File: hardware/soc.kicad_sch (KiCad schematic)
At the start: 2 parts, among them U16 MPFS025T-FCVG484E, U4 MPFS025T-FCVG484E

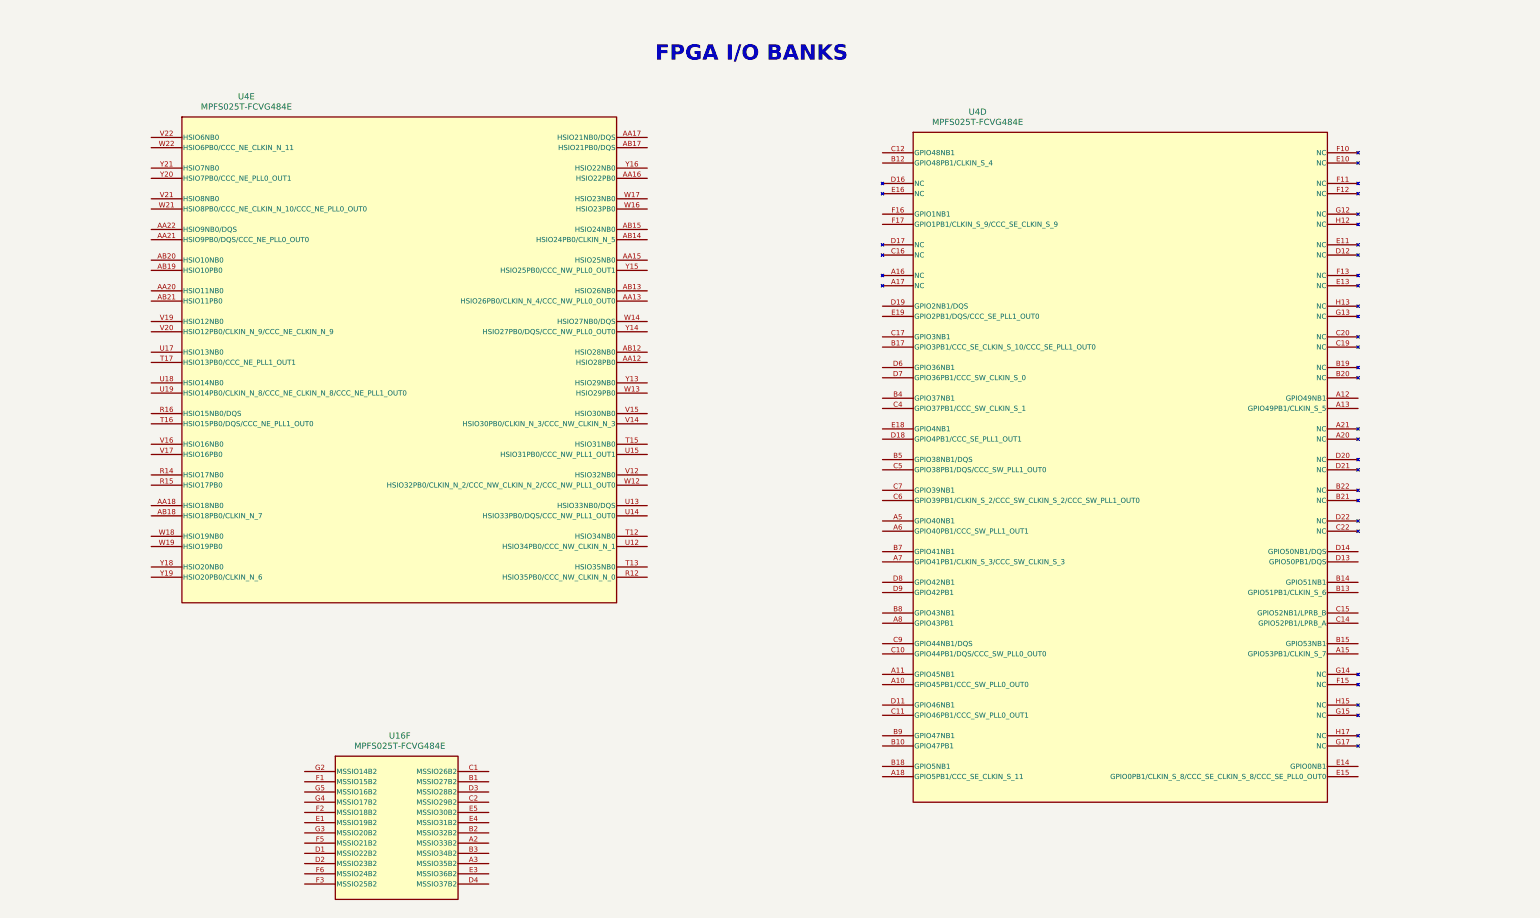
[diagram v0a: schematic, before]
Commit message: need finish io banks pinouts
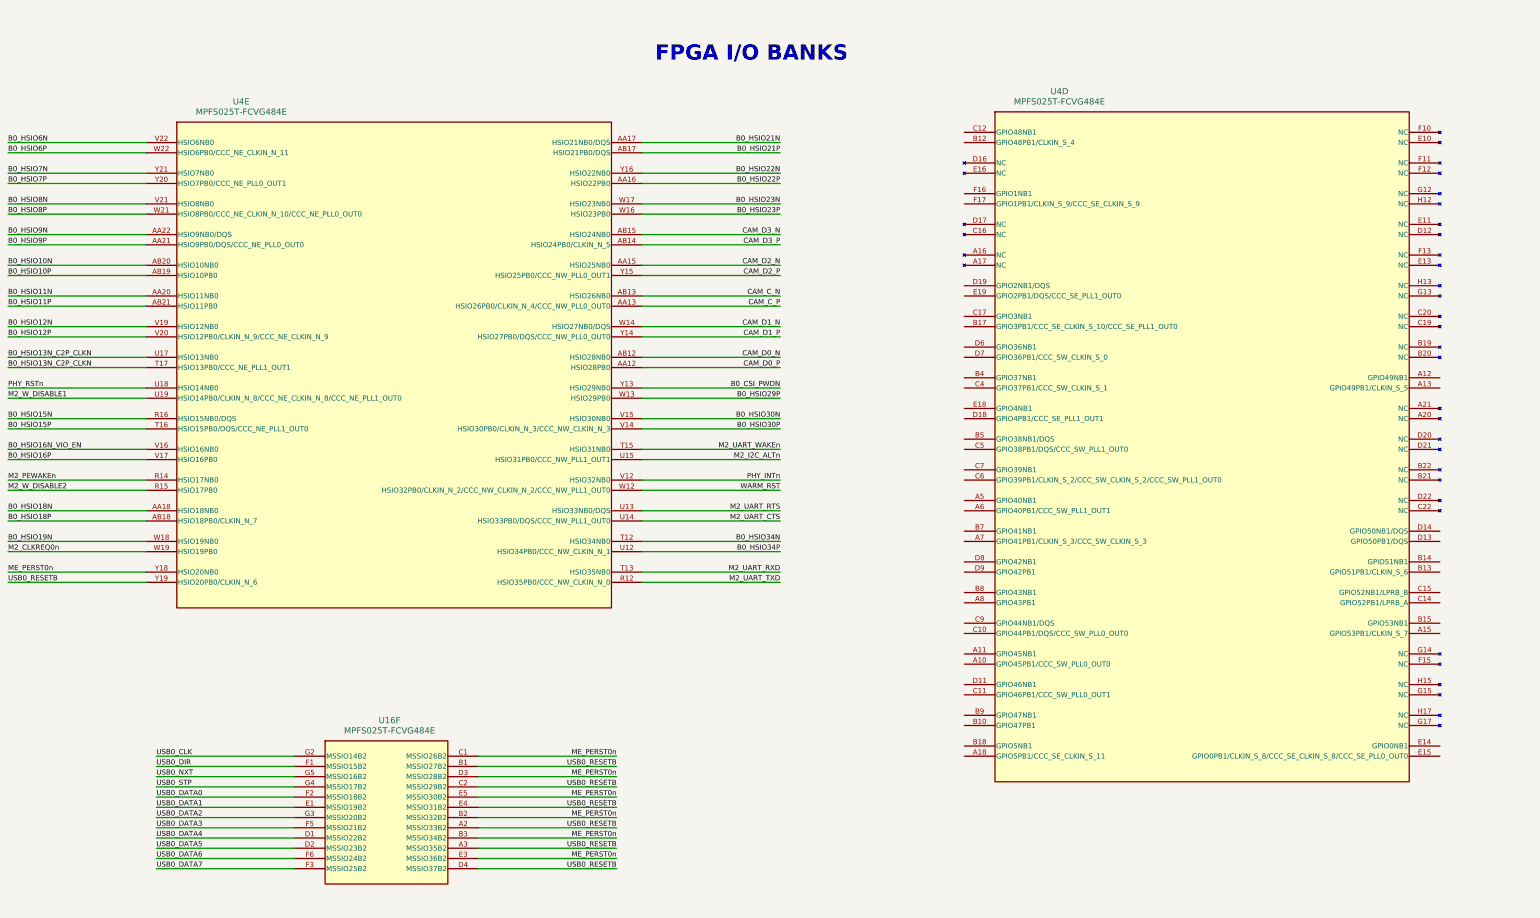
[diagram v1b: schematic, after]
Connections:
- net USB0_RESETB: now reaches U16.A2 (MSSIO33B2)
- net USB0_RESETB: now also U16.A3 (MSSIO35B2), U16.B1 (MSSIO27B2), U16.C2 (MSSIO29B2), U16.D4 (MSSIO37B2), U16.E4 (MSSIO31B2), U4.Y19 (HSIO20PB0/CLKIN_N_6)
- net ME_PERST0n: now reaches U16.B2 (MSSIO32B2)
- net ME_PERST0n: now also U16.B3 (MSSIO34B2), U16.C1 (MSSIO26B2), U16.D3 (MSSIO28B2), U16.E3 (MSSIO36B2), U16.E5 (MSSIO30B2), U4.Y18 (HSIO20NB0)
- net USB0_DATA4: now reaches U16.D1 (MSSIO22B2)
- net USB0_DATA5: now reaches U16.D2 (MSSIO23B2)
- net USB0_DATA1: now reaches U16.E1 (MSSIO19B2)
- net USB0_DIR: now reaches U16.F1 (MSSIO15B2)
- net USB0_DATA0: now reaches U16.F2 (MSSIO18B2)
- net USB0_DATA7: now reaches U16.F3 (MSSIO25B2)
- net USB0_DATA3: now reaches U16.F5 (MSSIO21B2)
- net USB0_DATA6: now reaches U16.F6 (MSSIO24B2)
- net USB0_CLK: now reaches U16.G2 (MSSIO14B2)
- net USB0_DATA2: now reaches U16.G3 (MSSIO20B2)
- net USB0_STP: now reaches U16.G4 (MSSIO17B2)
- net USB0_NXT: now reaches U16.G5 (MSSIO16B2)
- net CAM_D0_P: now reaches U4.AA12 (HSIO28PB0)
- net CAM_C_P: now reaches U4.AA13 (HSIO26PB0/CLKIN_N_4/CCC_NW_PLL0_OUT0)
- net CAM_D2_N: now reaches U4.AA15 (HSIO25NB0)
- net B0_HSIO22P: now reaches U4.AA16 (HSIO22PB0)
- net B0_HSIO21N: now reaches U4.AA17 (HSIO21NB0/DQS)
- net B0_HSIO18N: now reaches U4.AA18 (HSIO18NB0)
- net B0_HSIO11N: now reaches U4.AA20 (HSIO11NB0)
- net B0_HSIO9P: now reaches U4.AA21 (HSIO9PB0/DQS/CCC_NE_PLL0_OUT0)
- net B0_HSIO9N: now reaches U4.AA22 (HSIO9NB0/DQS)
- net CAM_D0_N: now reaches U4.AB12 (HSIO28NB0)
- net CAM_C_N: now reaches U4.AB13 (HSIO26NB0)
- net CAM_D3_P: now reaches U4.AB14 (HSIO24PB0/CLKIN_N_5)
- net CAM_D3_N: now reaches U4.AB15 (HSIO24NB0)
- net B0_HSIO21P: now reaches U4.AB17 (HSIO21PB0/DQS)
- net B0_HSIO18P: now reaches U4.AB18 (HSIO18PB0/CLKIN_N_7)
- net B0_HSIO10P: now reaches U4.AB19 (HSIO10PB0)
- net B0_HSIO10N: now reaches U4.AB20 (HSIO10NB0)
- net B0_HSIO11P: now reaches U4.AB21 (HSIO11PB0)
- net M2_UART_TXD: now reaches U4.R12 (HSIO35PB0/CCC_NW_CLKIN_N_0)
- net M2_PEWAKEn: now reaches U4.R14 (HSIO17NB0)
- net M2_W_DISABLE2: now reaches U4.R15 (HSIO17PB0)
- net B0_HSIO15N: now reaches U4.R16 (HSIO15NB0/DQS)
- net B0_HSIO34N: now reaches U4.T12 (HSIO34NB0)
- net M2_UART_RXD: now reaches U4.T13 (HSIO35NB0)
- net M2_UART_WAKEn: now reaches U4.T15 (HSIO31NB0)
- net B0_HSIO15P: now reaches U4.T16 (HSIO15PB0/DQS/CCC_NE_PLL1_OUT0)
- net B0_HSIO13N_C2P_CLKN: now reaches U4.T17 (HSIO13PB0/CCC_NE_PLL1_OUT1)
- net B0_HSIO13N_C2P_CLKN: now also U4.U17 (HSIO13NB0)
- net B0_HSIO34P: now reaches U4.U12 (HSIO34PB0/CCC_NW_CLKIN_N_1)
- net M2_UART_RTS: now reaches U4.U13 (HSIO33NB0/DQS)
- net M2_UART_CTS: now reaches U4.U14 (HSIO33PB0/DQS/CCC_NW_PLL1_OUT0)
- net M2_I2C_ALTn: now reaches U4.U15 (HSIO31PB0/CCC_NW_PLL1_OUT1)
- net PHY_RSTn: now reaches U4.U18 (HSIO14NB0)
- net M2_W_DISABLE1: now reaches U4.U19 (HSIO14PB0/CLKIN_N_8/CCC_NE_CLKIN_N_8/CCC_NE_PLL1_OUT0)
- net PHY_INTn: now reaches U4.V12 (HSIO32NB0)
- net B0_HSIO30P: now reaches U4.V14 (HSIO30PB0/CLKIN_N_3/CCC_NW_CLKIN_N_3)
- net B0_HSIO30N: now reaches U4.V15 (HSIO30NB0)
- net B0_HSIO16N_VIO_EN: now reaches U4.V16 (HSIO16NB0)
- net B0_HSIO16P: now reaches U4.V17 (HSIO16PB0)
- net B0_HSIO12N: now reaches U4.V19 (HSIO12NB0)
- net B0_HSIO12P: now reaches U4.V20 (HSIO12PB0/CLKIN_N_9/CCC_NE_CLKIN_N_9)
- net B0_HSIO8N: now reaches U4.V21 (HSIO8NB0)
- net B0_HSIO6N: now reaches U4.V22 (HSIO6NB0)
- net WARM_RST: now reaches U4.W12 (HSIO32PB0/CLKIN_N_2/CCC_NW_CLKIN_N_2/CCC_NW_PLL1_OUT0)
- net B0_HSIO29P: now reaches U4.W13 (HSIO29PB0)
- net CAM_D1_N: now reaches U4.W14 (HSIO27NB0/DQS)
- net B0_HSIO23P: now reaches U4.W16 (HSIO23PB0)
- net B0_HSIO23N: now reaches U4.W17 (HSIO23NB0)
- net B0_HSIO19N: now reaches U4.W18 (HSIO19NB0)
- net M2_CLKREQ0n: now reaches U4.W19 (HSIO19PB0)
- net B0_HSIO8P: now reaches U4.W21 (HSIO8PB0/CCC_NE_CLKIN_N_10/CCC_NE_PLL0_OUT0)
- net B0_HSIO6P: now reaches U4.W22 (HSIO6PB0/CCC_NE_CLKIN_N_11)
- net B0_CSI_PWDN: now reaches U4.Y13 (HSIO29NB0)
- net CAM_D1_P: now reaches U4.Y14 (HSIO27PB0/DQS/CCC_NW_PLL0_OUT0)
- net CAM_D2_P: now reaches U4.Y15 (HSIO25PB0/CCC_NW_PLL0_OUT1)
- net B0_HSIO22N: now reaches U4.Y16 (HSIO22NB0)
- net B0_HSIO7P: now reaches U4.Y20 (HSIO7PB0/CCC_NE_PLL0_OUT1)
- net B0_HSIO7N: now reaches U4.Y21 (HSIO7NB0)
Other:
- moved on the sheet: U16F, U4D, U4E

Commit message: updated hardware
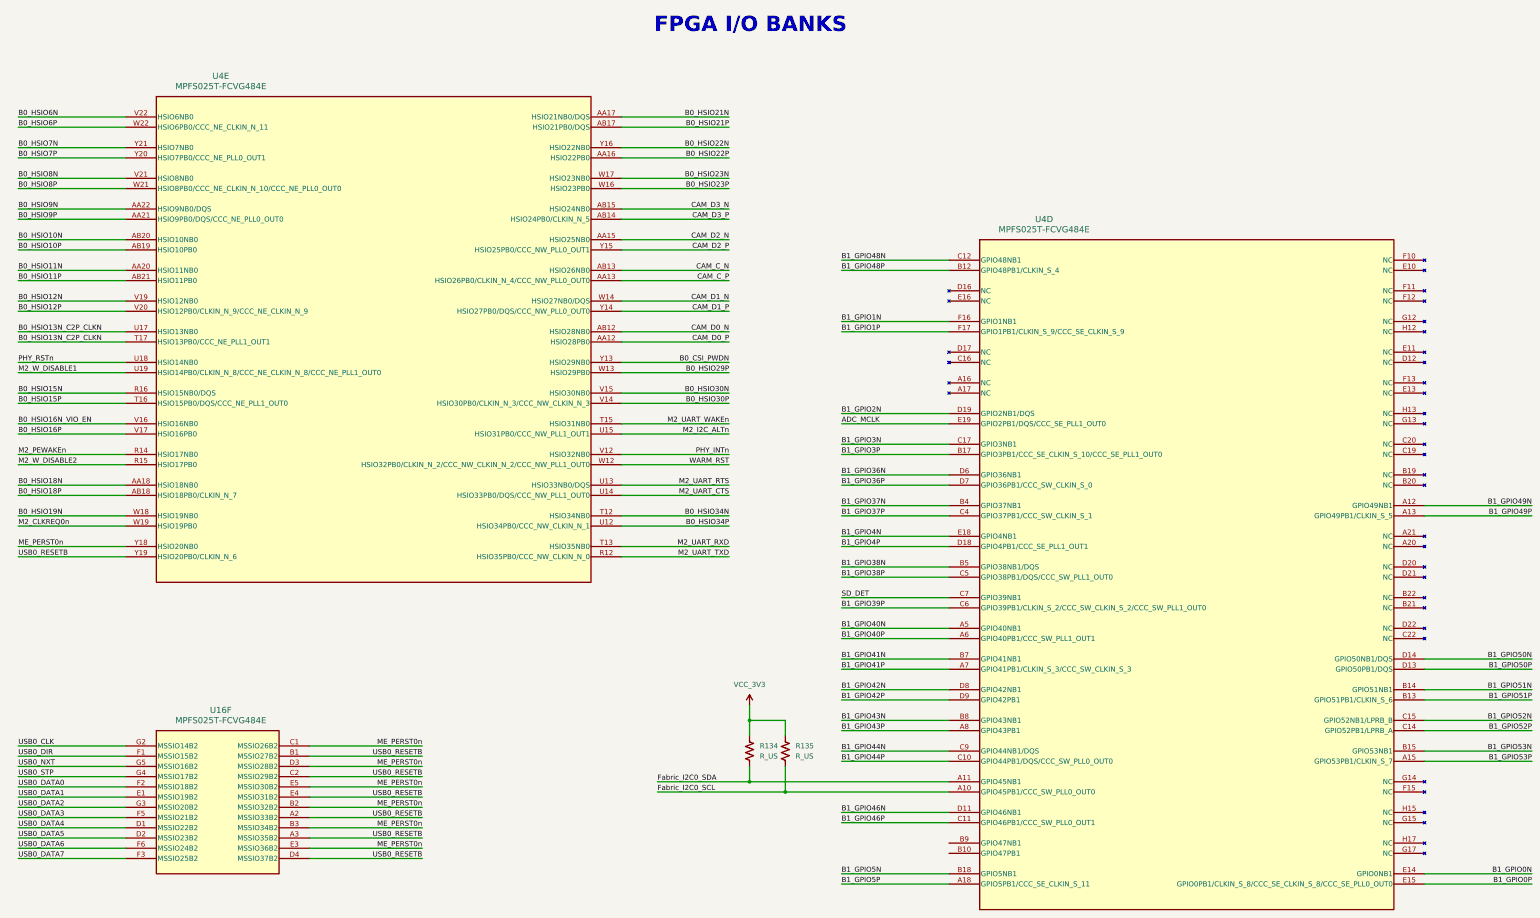
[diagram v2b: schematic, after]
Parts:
- added R134, R135: R_US, symbol Device:R_US
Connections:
- net Fabric_I2C0_SCL: now reaches U4.A10 (GPIO45PB1/CCC_SW_PLL0_OUT0)
- net Fabric_I2C0_SCL: now also R135.2
- net Fabric_I2C0_SDA: now reaches U4.A11 (GPIO45NB1)
- net Fabric_I2C0_SDA: now also R134.2
- net B1_GPIO49N: now reaches U4.A12 (GPIO49NB1)
- net B1_GPIO49P: now reaches U4.A13 (GPIO49PB1/CLKIN_S_5)
- net B1_GPIO53P: now reaches U4.A15 (GPIO53PB1/CLKIN_S_7)
- net B1_GPIO5P: now reaches U4.A18 (GPIO5PB1/CCC_SE_CLKIN_S_11)
- net B1_GPIO40N: now reaches U4.A5 (GPIO40NB1)
- net B1_GPIO40P: now reaches U4.A6 (GPIO40PB1/CCC_SW_PLL1_OUT1)
- net B1_GPIO41P: now reaches U4.A7 (GPIO41PB1/CLKIN_S_3/CCC_SW_CLKIN_S_3)
- net B1_GPIO43P: now reaches U4.A8 (GPIO43PB1)
- net B1_GPIO48P: now reaches U4.B12 (GPIO48PB1/CLKIN_S_4)
- net B1_GPIO51P: now reaches U4.B13 (GPIO51PB1/CLKIN_S_6)
- net B1_GPIO51N: now reaches U4.B14 (GPIO51NB1)
- net B1_GPIO53N: now reaches U4.B15 (GPIO53NB1)
- net B1_GPIO3P: now reaches U4.B17 (GPIO3PB1/CCC_SE_CLKIN_S_10/CCC_SE_PLL1_OUT0)
- net B1_GPIO5N: now reaches U4.B18 (GPIO5NB1)
- net B1_GPIO37N: now reaches U4.B4 (GPIO37NB1)
- net B1_GPIO38N: now reaches U4.B5 (GPIO38NB1/DQS)
- net B1_GPIO41N: now reaches U4.B7 (GPIO41NB1)
- net B1_GPIO43N: now reaches U4.B8 (GPIO43NB1)
- net B1_GPIO44P: now reaches U4.C10 (GPIO44PB1/DQS/CCC_SW_PLL0_OUT0)
- net B1_GPIO46P: now reaches U4.C11 (GPIO46PB1/CCC_SW_PLL0_OUT1)
- net B1_GPIO48N: now reaches U4.C12 (GPIO48NB1)
- net B1_GPIO52P: now reaches U4.C14 (GPIO52PB1/LPRB_A)
- net B1_GPIO52N: now reaches U4.C15 (GPIO52NB1/LPRB_B)
- net B1_GPIO3N: now reaches U4.C17 (GPIO3NB1)
- net B1_GPIO37P: now reaches U4.C4 (GPIO37PB1/CCC_SW_CLKIN_S_1)
- net B1_GPIO38P: now reaches U4.C5 (GPIO38PB1/DQS/CCC_SW_PLL1_OUT0)
- net B1_GPIO39P: now reaches U4.C6 (GPIO39PB1/CLKIN_S_2/CCC_SW_CLKIN_S_2/CCC_SW_PLL1_OUT0)
- net SD_DET: now reaches U4.C7 (GPIO39NB1)
- net B1_GPIO44N: now reaches U4.C9 (GPIO44NB1/DQS)
- net B1_GPIO46N: now reaches U4.D11 (GPIO46NB1)
- net B1_GPIO50P: now reaches U4.D13 (GPIO50PB1/DQS)
- net B1_GPIO50N: now reaches U4.D14 (GPIO50NB1/DQS)
- net B1_GPIO4P: now reaches U4.D18 (GPIO4PB1/CCC_SE_PLL1_OUT1)
- net B1_GPIO2N: now reaches U4.D19 (GPIO2NB1/DQS)
- net B1_GPIO36N: now reaches U4.D6 (GPIO36NB1)
- net B1_GPIO36P: now reaches U4.D7 (GPIO36PB1/CCC_SW_CLKIN_S_0)
- net B1_GPIO42N: now reaches U4.D8 (GPIO42NB1)
- net B1_GPIO42P: now reaches U4.D9 (GPIO42PB1)
- net B1_GPIO0N: now reaches U4.E14 (GPIO0NB1)
- net B1_GPIO0P: now reaches U4.E15 (GPIO0PB1/CLKIN_S_8/CCC_SE_CLKIN_S_8/CCC_SE_PLL0_OUT0)
- net B1_GPIO4N: now reaches U4.E18 (GPIO4NB1)
- net ADC_MCLK: now reaches U4.E19 (GPIO2PB1/DQS/CCC_SE_PLL1_OUT0)
- net B1_GPIO1N: now reaches U4.F16 (GPIO1NB1)
- net B1_GPIO1P: now reaches U4.F17 (GPIO1PB1/CLKIN_S_9/CCC_SE_CLKIN_S_9)
- new net VCC_3V3: R134.1, R135.1
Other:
- moved on the sheet: U16F, U4D, U4E
